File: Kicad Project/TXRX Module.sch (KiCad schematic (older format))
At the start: 19 parts, among them U10 GALI-2+, U11 BandpassFilter, U12 ufl, U13 Antenna111, U14 Antenna111, U15 ufl, U3 BandpassFilter, U9 LEE-39+

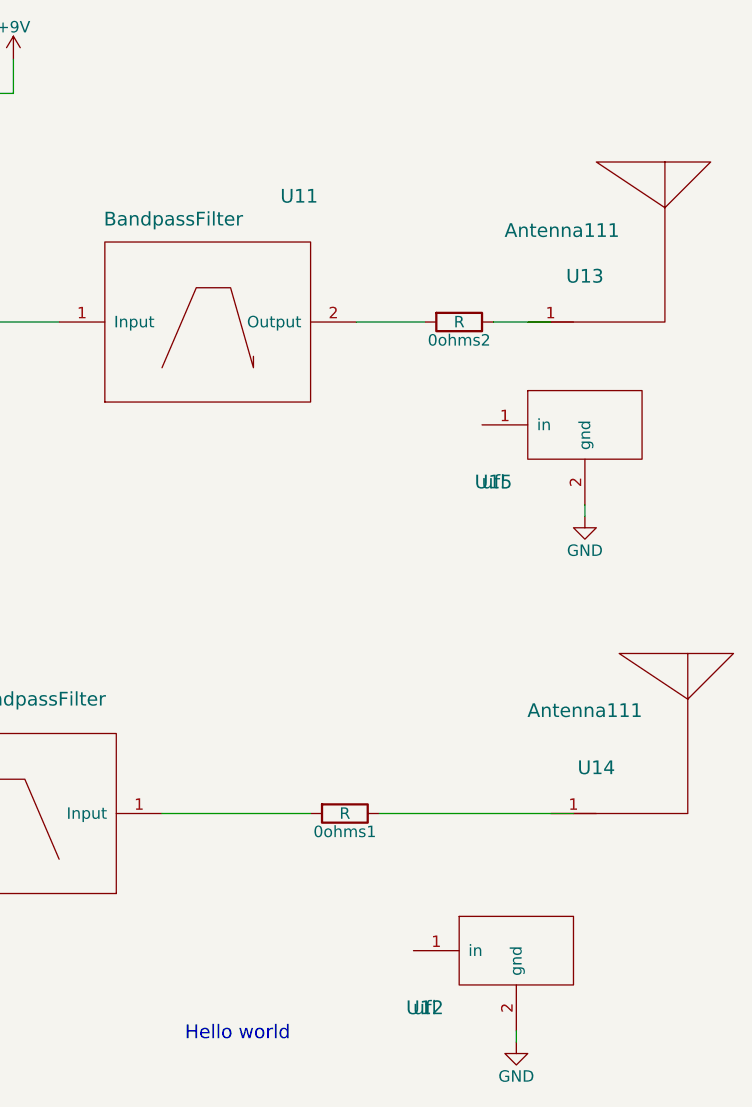
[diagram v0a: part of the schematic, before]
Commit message: PCB Changes
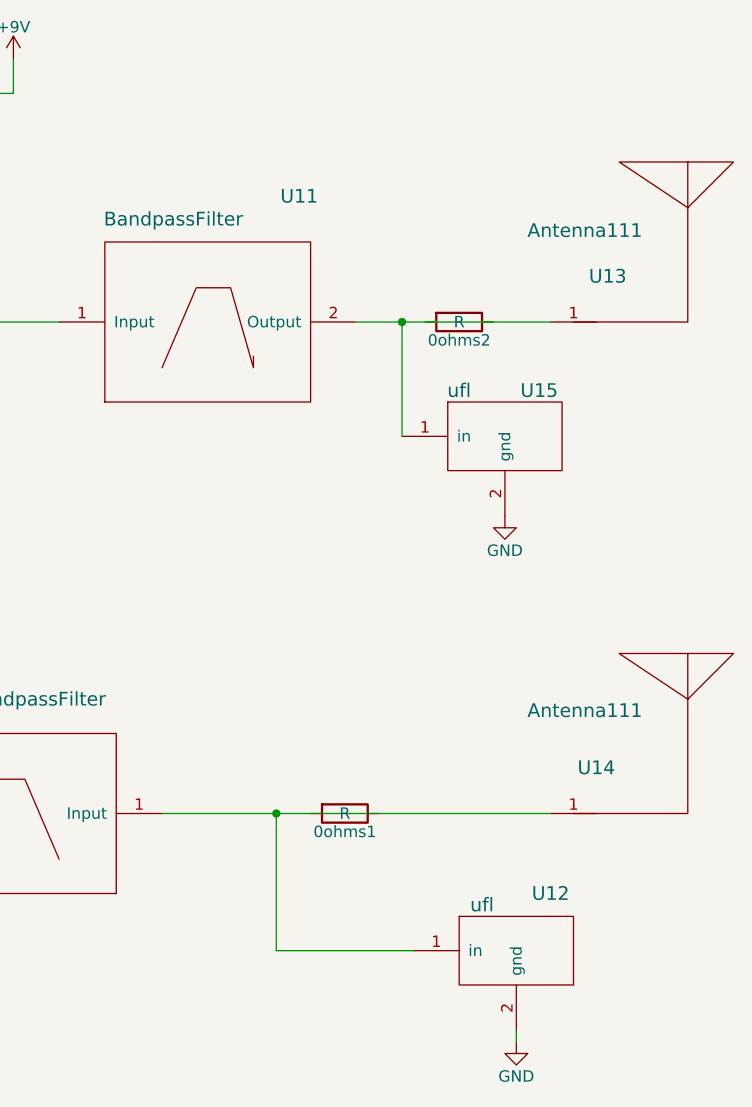
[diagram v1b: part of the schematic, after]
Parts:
- 0ohms1, 0ohms2: footprint (none) -> RadarComponents:100PAD
- C12, R18, R19: footprint RadarComponents:100PAD -> RadarComponents:100PAD+GND2
- U12, U15: footprint (none) -> RadarComponents:UFL
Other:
- note removed: "Hello world"
- moved on the sheet: U13, U15
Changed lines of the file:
@@
 Comment4 ""
 $EndDescr
-Text Notes 6500 5800 0    60   ~ 0
-Hello world
 $Comp
 L C C11
@@
 F 0 "R19" V 5580 1650 50  0000 C CNN
 F 1 "75" V 5500 1650 50  0000 C CNN
-F 2 "RadarComponents:100PAD" V 5430 1650 50  0001 C CNN
+F 2 "RadarComponents:100PAD+GND2" V 5430 1650 50  0001 C CNN
 F 3 "" H 5500 1650 50  0001 C CNN
 	1    5500 1650
@@
 F 0 "C12" H 2675 4300 50  0000 L CNN
 F 1 "150p" H 2675 4100 50  0000 L CNN
-F 2 "RadarComponents:100PAD" H 2688 4050 50  0001 C CNN
+F 2 "RadarComponents:100PAD+GND2" H 2688 4050 50  0001 C CNN
 F 3 "" H 2650 4200 50  0001 C CNN
 	1    2650 4200
@@
 L Antenna111 U13
 U 1 1 59FFCB61
-P 7400 3000
-F 0 "U13" H 8250 3550 60  0000 C CNN
-F 1 "Antenna111" H 8150 3750 60  0000 C CNN
-F 2 "RadarComponents:patch58" H 7400 3000 60  0001 C CNN
-F 3 "" H 7400 3000 60  0001 C CNN
-	1    7400 3000
+P 7500 3000
+F 0 "U13" H 8350 3550 60  0000 C CNN
+F 1 "Antenna111" H 8250 3750 60  0000 C CNN
+F 2 "RadarComponents:patch58" H 7500 3000 60  0001 C CNN
+F 3 "" H 7500 3000 60  0001 C CNN
+	1    7500 3000
 	1    0    0    -1
 $EndComp
@@
 F 0 "R18" V 5030 2450 50  0000 C CNN
 F 1 "75" V 4950 2450 50  0000 C CNN
-F 2 "RadarComponents:100PAD" V 4880 2450 50  0001 C CNN
+F 2 "RadarComponents:100PAD+GND2" V 4880 2450 50  0001 C CNN
 F 3 "" H 4950 2450 50  0001 C CNN
 	1    4950 2450
 	1    0    0    -1
 $EndComp
-Wire Wire Line
-	2350 2650 2700 2650
-Wire Wire Line
-	3000 2650 3350 2650
-Wire Wire Line
-	4750 2650 5150 2650
-Wire Wire Line
-	5450 2650 5950 2650
-Wire Wire Line
-	4950 2600 4950 2650
-Connection ~ 4950 2650
-Wire Wire Line
-	4950 1650 4950 2300
-Wire Wire Line
-	4950 2100 5150 2100
-Wire Wire Line
-	4950 1650 5350 1650
-Connection ~ 4950 2100
 $Comp
 L R R17
@@
 $EndComp
 $Comp
-L GND #PWR010
+L GND #PWR011
 U 1 1 59FFE5A2
 P 2350 4350
-F 0 "#PWR010" H 2350 4100 50  0001 C CNN
+F 0 "#PWR011" H 2350 4100 50  0001 C CNN
 F 1 "GND" H 2350 4200 50  0000 C CNN
 F 2 "" H 2350 4350 50  0001 C CNN
@@
 $EndComp
 $Comp
-L GND #PWR011
+L GND #PWR012
 U 1 1 59FFE5D4
 P 3850 5400
-F 0 "#PWR011" H 3850 5150 50  0001 C CNN
+F 0 "#PWR012" H 3850 5150 50  0001 C CNN
 F 1 "GND" H 3850 5250 50  0000 C CNN
 F 2 "" H 3850 5400 50  0001 C CNN
@@
 $EndComp
 $Comp
-L GND #PWR012
+L GND #PWR013
 U 1 1 59FFE606
 P 4050 3200
-F 0 "#PWR012" H 4050 2950 50  0001 C CNN
+F 0 "#PWR013" H 4050 2950 50  0001 C CNN
 F 1 "GND" H 4050 3050 50  0000 C CNN
 F 2 "" H 4050 3200 50  0001 C CNN
@@
 $EndComp
 $Comp
-L GND #PWR013
+L GND #PWR014
 U 1 1 59FFE638
 P 5450 2200
-F 0 "#PWR013" H 5450 1950 50  0001 C CNN
+F 0 "#PWR014" H 5450 1950 50  0001 C CNN
 F 1 "GND" H 5450 2050 50  0000 C CNN
 F 2 "" H 5450 2200 50  0001 C CNN
@@
 	1    0    0    -1
 $EndComp
-Wire Wire Line
-	2850 4800 3150 4800
-Wire Wire Line
-	2950 4750 2950 4800
-Connection ~ 2950 4800
-Wire Wire Line
-	2950 3950 2950 4450
-Wire Wire Line
-	2950 3950 3300 3950
-Wire Wire Line
-	2800 4200 2950 4200
-Connection ~ 2950 4200
-Wire Wire Line
-	2500 4200 2350 4200
-Wire Wire Line
-	2350 4200 2350 4350
-Wire Wire Line
-	3850 5250 3850 5400
-Wire Wire Line
-	5450 2100 5450 2200
-Wire Wire Line
-	4050 3100 4050 3200
-Wire Wire Line
-	2350 4800 2550 4800
-$Comp
-L +9V #PWR014
+$Comp
+L +9V #PWR015
 U 1 1 5A01141C
 P 5750 1500
-F 0 "#PWR014" H 5750 1350 50  0001 C CNN
+F 0 "#PWR015" H 5750 1350 50  0001 C CNN
 F 1 "+9V" H 5750 1640 50  0000 C CNN
 F 2 "" H 5750 1500 50  0001 C CNN
@@
 $EndComp
 $Comp
-L +9V #PWR015
+L +9V #PWR016
 U 1 1 5A0114D0
 P 3700 3800
-F 0 "#PWR015" H 3700 3650 50  0001 C CNN
+F 0 "#PWR016" H 3700 3650 50  0001 C CNN
 F 1 "+9V" H 3700 3940 50  0000 C CNN
 F 2 "" H 3700 3800 50  0001 C CNN
@@
 	1    0    0    -1
 $EndComp
-Wire Wire Line
-	3600 3950 3700 3950
-Wire Wire Line
-	3700 3950 3700 3800
-Wire Wire Line
-	5650 1650 5750 1650
-Wire Wire Line
-	5750 1650 5750 1500
-Wire Wire Line
-	4550 4800 5100 4800
 Text GLabel 2350 2650 0    60   Input ~ 0
 PowerSplitter
@@
 F 0 "0ohms1" V 7280 4800 50  0000 C CNN
 F 1 "R" V 7200 4800 50  0000 C CNN
-F 2 "" V 7130 4800 50  0001 C CNN
+F 2 "RadarComponents:100PAD" V 7130 4800 50  0001 C CNN
 F 3 "" H 7200 4800 50  0001 C CNN
 	1    7200 4800
@@
 F 0 "0ohms2" V 7780 2650 50  0000 C CNN
 F 1 "R" V 7700 2650 50  0000 C CNN
-F 2 "" V 7630 2650 50  0001 C CNN
+F 2 "RadarComponents:100PAD" V 7630 2650 50  0001 C CNN
 F 3 "" H 7700 2650 50  0001 C CNN
 	1    7700 2650
 	0    1    1    0
 $EndComp
-Wire Wire Line
-	8200 4800 7350 4800
-Wire Wire Line
-	6400 4800 7050 4800
-Wire Wire Line
-	7550 2650 7250 2650
-Wire Wire Line
-	8100 2650 7850 2650
 $Comp
 L ufl U15
 U 1 1 5A0330EA
-P 7850 3350
-F 0 "U15" H 7850 3350 60  0000 C CNN
-F 1 "ufl" H 7850 3350 60  0000 C CNN
-F 2 "" H 7850 3350 60  0001 C CNN
-F 3 "" H 7850 3350 60  0001 C CNN
-	1    7850 3350
+P 7500 3400
+F 0 "U15" H 8050 3850 60  0000 C CNN
+F 1 "ufl" H 7700 3850 60  0000 C CNN
+F 2 "RadarComponents:UFL" H 7500 3400 60  0001 C CNN
+F 3 "" H 7500 3400 60  0001 C CNN
+	1    7500 3400
 	1    0    0    -1
 $EndComp
@@
 U 1 1 5A0331E6
 P 7550 5650
-F 0 "U12" H 7550 5650 60  0000 C CNN
-F 1 "ufl" H 7550 5650 60  0000 C CNN
-F 2 "" H 7550 5650 60  0001 C CNN
+F 0 "U12" H 8100 6150 60  0000 C CNN
+F 1 "ufl" H 7800 6100 60  0000 C CNN
+F 2 "RadarComponents:UFL" H 7550 5650 60  0001 C CNN
 F 3 "" H 7550 5650 60  0001 C CNN
 	1    7550 5650
@@
 $EndComp
 $Comp
-L GND #PWR016
+L GND #PWR017
 U 1 1 5A03325F
-P 8250 3500
-F 0 "#PWR016" H 8250 3250 50  0001 C CNN
-F 1 "GND" H 8250 3350 50  0000 C CNN
-F 2 "" H 8250 3500 50  0001 C CNN
-F 3 "" H 8250 3500 50  0001 C CNN
-	1    8250 3500
-	1    0    0    -1
-$EndComp
-$Comp
-L GND #PWR017
+P 7900 3500
+F 0 "#PWR017" H 7900 3250 50  0001 C CNN
+F 1 "GND" H 7900 3350 50  0000 C CNN
+F 2 "" H 7900 3500 50  0001 C CNN
+F 3 "" H 7900 3500 50  0001 C CNN
+	1    7900 3500
+	1    0    0    -1
+$EndComp
+$Comp
+L GND #PWR018
 U 1 1 5A03329B
 P 7950 5800
-F 0 "#PWR017" H 7950 5550 50  0001 C CNN
+F 0 "#PWR018" H 7950 5550 50  0001 C CNN
 F 1 "GND" H 7950 5650 50  0000 C CNN
 F 2 "" H 7950 5800 50  0001 C CNN
@@
 $EndComp
 Wire Wire Line
+	2350 2650 2700 2650
+Wire Wire Line
+	3000 2650 3350 2650
+Wire Wire Line
+	4750 2650 5150 2650
+Wire Wire Line
+	5450 2650 5950 2650
+Wire Wire Line
+	4950 2600 4950 2650
+Connection ~ 4950 2650
+Wire Wire Line
+	4950 1650 4950 2300
+Wire Wire Line
+	4950 2100 5150 2100
+Wire Wire Line
+	4950 1650 5350 1650
+Connection ~ 4950 2100
+Wire Wire Line
+	2850 4800 3150 4800
+Wire Wire Line
+	2950 4750 2950 4800
+Connection ~ 2950 4800
+Wire Wire Line
+	2950 3950 2950 4450
+Wire Wire Line
+	2950 3950 3300 3950
+Wire Wire Line
+	2800 4200 2950 4200
+Connection ~ 2950 4200
+Wire Wire Line
+	2500 4200 2350 4200
+Wire Wire Line
+	2350 4200 2350 4350
+Wire Wire Line
+	3850 5250 3850 5400
+Wire Wire Line
+	5450 2100 5450 2200
+Wire Wire Line
+	4050 3100 4050 3200
+Wire Wire Line
+	2350 4800 2550 4800
+Wire Wire Line
+	3600 3950 3700 3950
+Wire Wire Line
+	3700 3950 3700 3800
+Wire Wire Line
+	5650 1650 5750 1650
+Wire Wire Line
+	5750 1650 5750 1500
+Wire Wire Line
+	4550 4800 5100 4800
+Wire Wire Line
 	7950 5800 7950 5750
 Wire Wire Line
-	8250 3500 8250 3450
+	7450 3150 7450 2650
+Connection ~ 7450 2650
+Wire Wire Line
+	7500 5400 6900 5400
+Wire Wire Line
+	6900 5400 6900 4800
+Connection ~ 6900 4800
+Wire Wire Line
+	6400 4800 8100 4800
+Wire Wire Line
+	8100 2650 7250 2650
 $EndSCHEMATC
